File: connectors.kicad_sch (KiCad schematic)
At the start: 25 parts, among them J1 Conn_01x04_Pin, J13 Conn_01x06, J14 Conn_01x06, J16 Conn_01x06, J17 Conn_01x06, J2 USB_C_Receptacle_USB2.0_16P, J3 Conn_01x08, J4 Micro_SD_Card, J5 Conn_01x08, J6 Conn_01x03, J7 Conn_01x02, J8 Conn_01x05, J9 Conn_01x06, U9 USBLC6-2P6

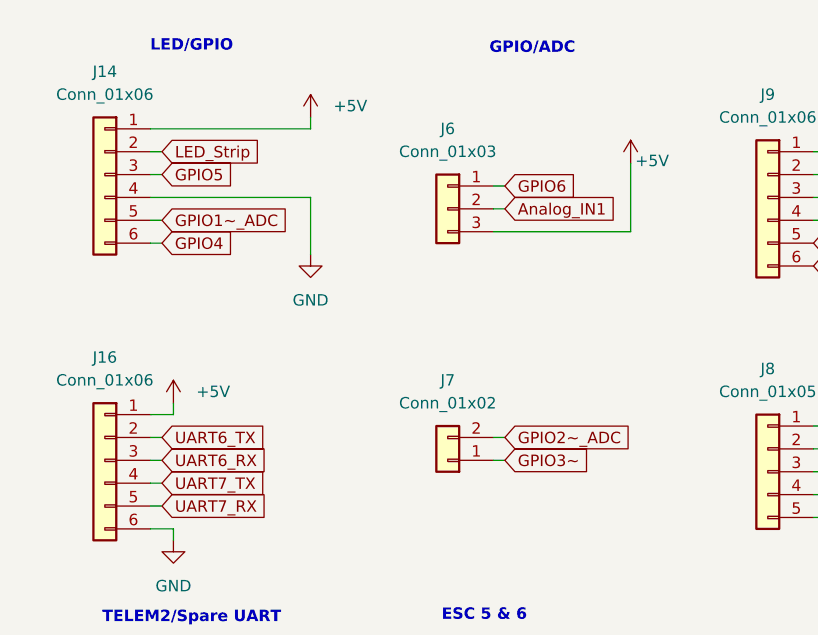
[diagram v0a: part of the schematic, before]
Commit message: Add V1.1
Add V1.1

Add V1.1
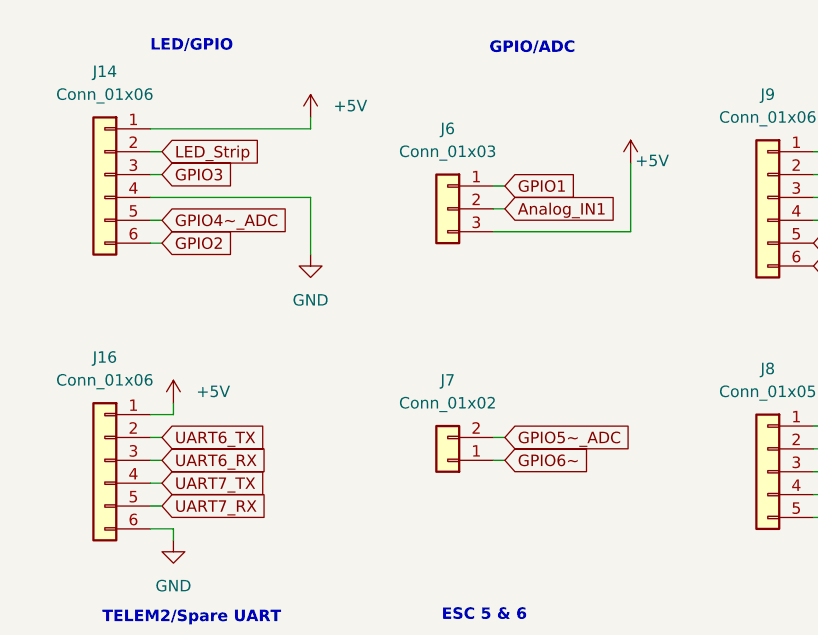
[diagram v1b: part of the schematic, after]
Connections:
- net GPIO1~_ADC renamed GPIO4~_ADC
- net GPIO2~_ADC renamed GPIO5~_ADC
- net GPIO3~ renamed GPIO6~
- net GPIO4 renamed GPIO2
- net GPIO5 renamed GPIO3
- net GPIO6 renamed GPIO1
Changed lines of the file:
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@@
 	(title_block
 		(title "STM32H5 FC")
-		(date "08/06/2026")
-		(rev "v1")
+		(date "2026-05-11")
+		(rev "v1.1")
 		(comment 1 "Evans Cesil Thomas")
 	)
@@
 		)
 	)
-	(global_label "GPIO4"
+	(global_label "GPIO2"
 		(shape input)
 		(at 138.43 96.52 0)
@@
 		)
 	)
-	(global_label "GPIO3~"
+	(global_label "GPIO6~"
 		(shape input)
 		(at 176.53 120.65 0)
@@
 		)
 	)
-	(global_label "GPIO6"
+	(global_label "GPIO1"
 		(shape input)
 		(at 176.53 90.17 0)
@@
 		)
 	)
-	(global_label "GPIO2~_ADC"
+	(global_label "GPIO5~_ADC"
 		(shape input)
 		(at 176.53 118.11 0)
@@
 		)
 	)
-	(global_label "GPIO5"
+	(global_label "GPIO3"
 		(shape input)
 		(at 138.43 88.9 0)
@@
 		)
 	)
-	(global_label "GPIO1~_ADC"
+	(global_label "GPIO4~_ADC"
 		(shape input)
 		(at 138.43 93.98 0)
